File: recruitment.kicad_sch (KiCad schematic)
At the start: 1 part

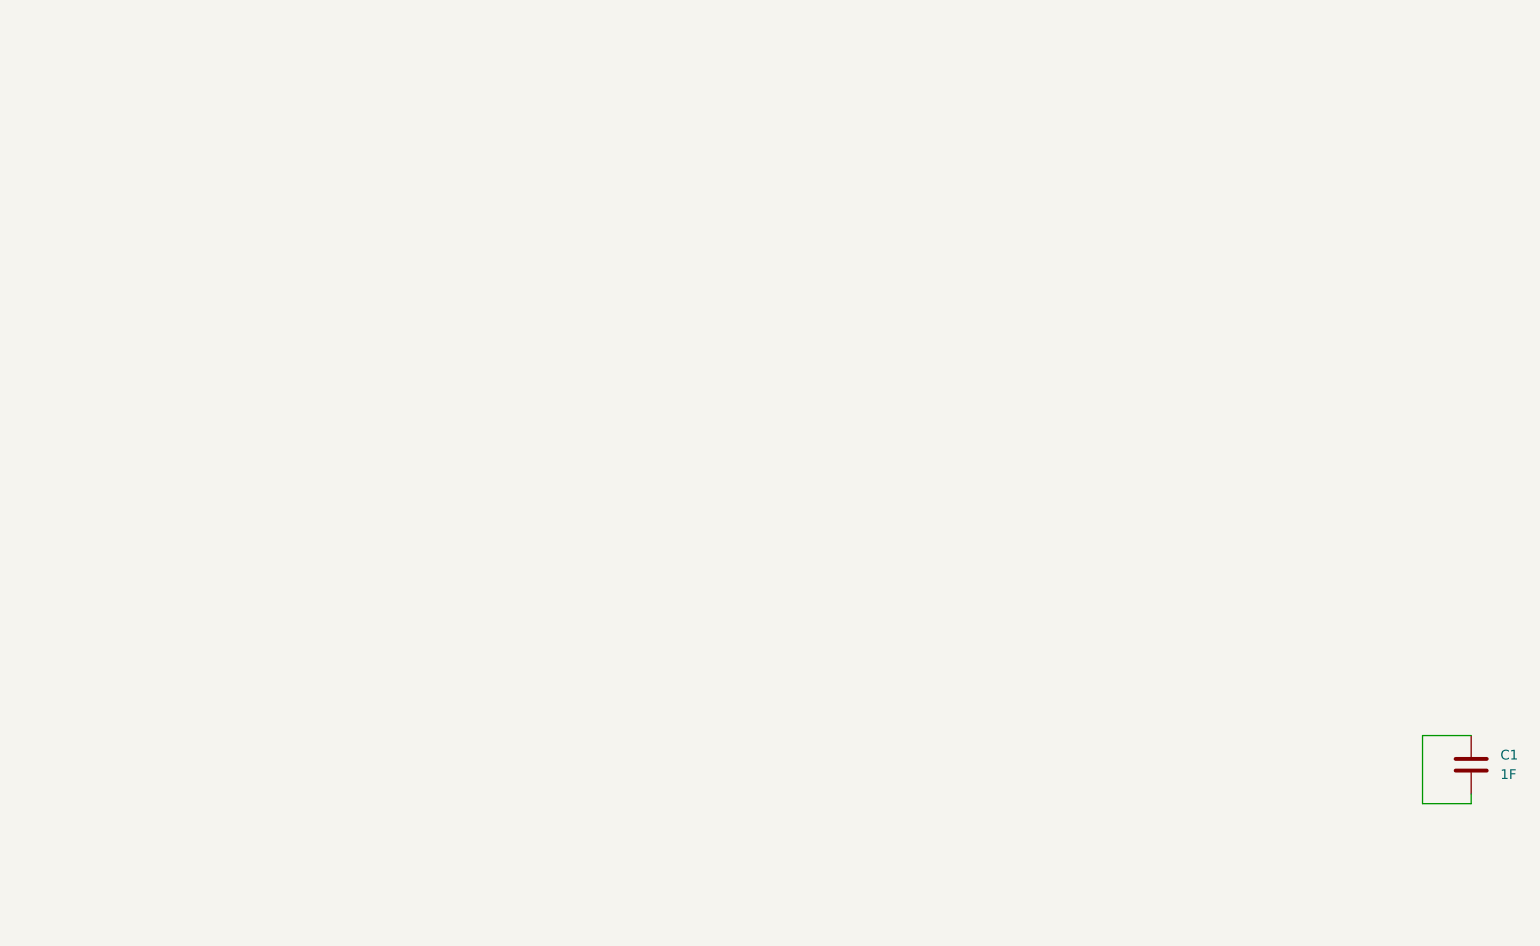
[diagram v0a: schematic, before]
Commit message: inizio progettazione circuito
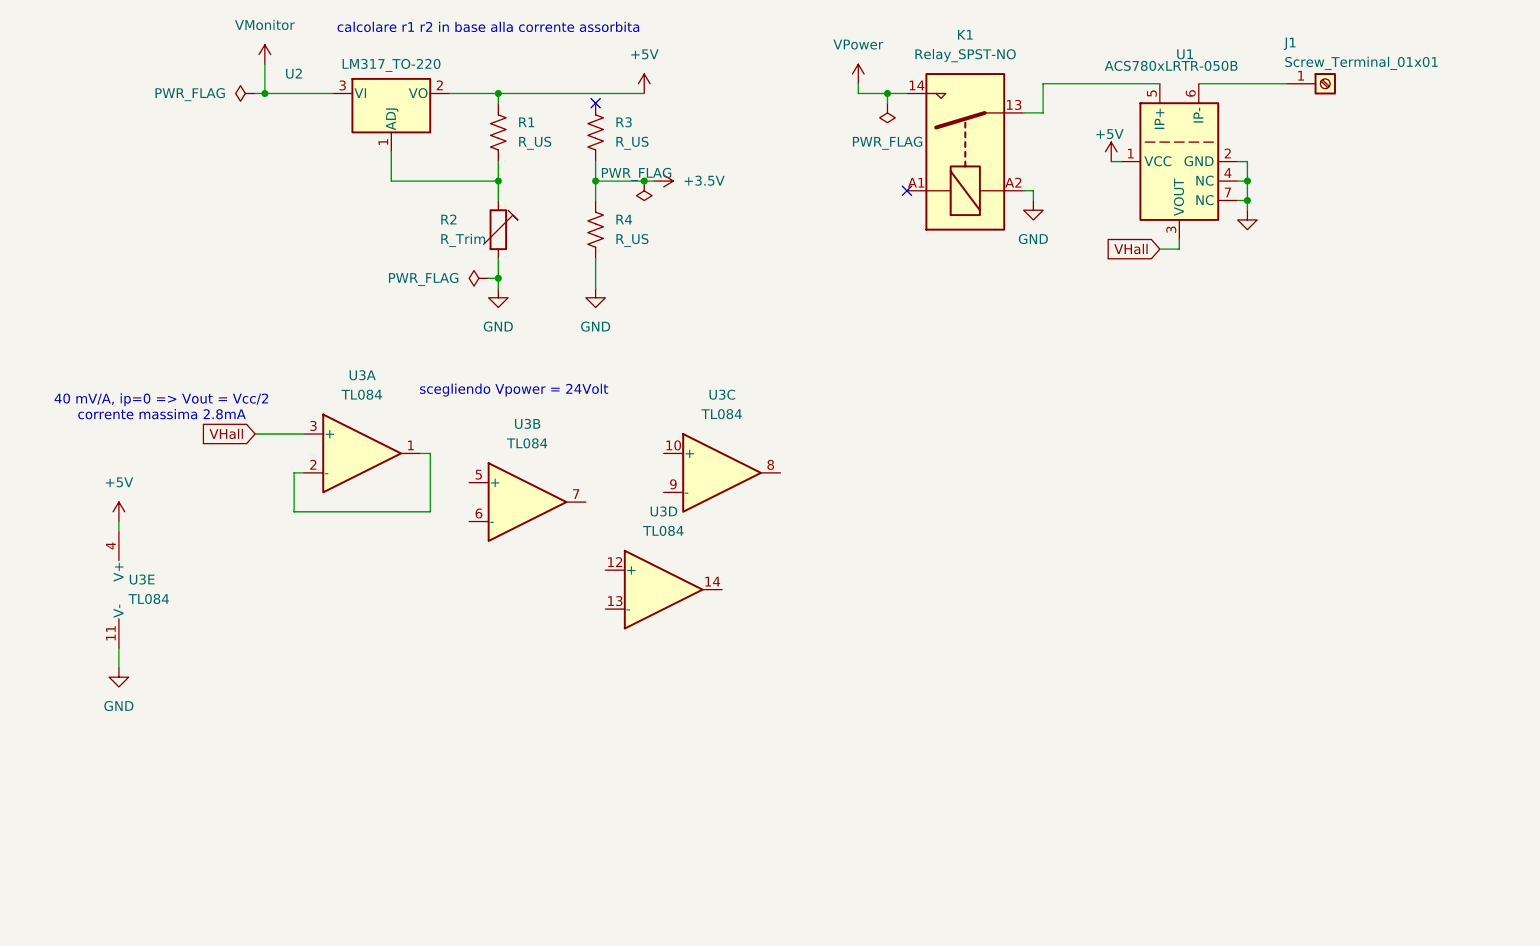
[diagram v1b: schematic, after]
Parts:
- removed C1: 1F, Capacitor_SMD:C_0805_2012Metric, symbol Device:C
- added J1: Screw_Terminal_01x01, TerminalBlock:TerminalBlock_Altech_AK300-2_P5.00mm, symbol Connector:Screw_Terminal_01x01
- added K1: Relay_SPST-NO, Relay_THT:Relay_1-Form-A_Schrack-RYII_RM5mm, symbol Relay:Relay_SPST-NO
- added R1, R3, R4: R_US, symbol Device:R_US
- added R2: R_Trim, symbol Device:R_Trim
- added U1: ACS780xLRTR-050B, Sensor_Current:Allegro_PSOF-7_4.8x6.4mm_P1.60mm, symbol Sensor_Current:ACS780xLRTR-050B
- added U2: LM317_TO-220, Package_TO_SOT_THT:TO-220-3_Vertical, symbol Regulator_Linear:LM317_TO-220
- added U3: TL084, symbol Amplifier_Operational:TL084
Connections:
- new net: R1.2, R2.1, U2.1 (ADJ)
- new net: J1.1 (Pin_1), U1.6 (IP-)
- new net: K1.13, U1.5 (IP+)
- new net: U3.1, U3.2 (-)
- new net +3.5V: R3.2, R4.1
- new net +5V: R1.1, U1.1 (VCC), U2.2 (VO), U3.4 (V+)
- new net GND: K1.A2, R2.2, R4.2, U1.2 (GND), U1.4 (NC), U1.7 (NC), U3.11 (V-)
- new net VHall: U1.3 (VOUT), U3.3 (+)
- new net VMonitor: U2.3 (VI)
- new net VPower: K1.14
- no-connect marks 0 -> 2
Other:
- note added: "40 mV/A, ip=0 => Vout = Vcc/2 corrente massima 2.8mA"
- note added: "calcolare r1 r2 in base alla corrente assorbita"
- note added: "scegliendo Vpower = 24Volt"

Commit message: giorno 2 : prime prove e footprint
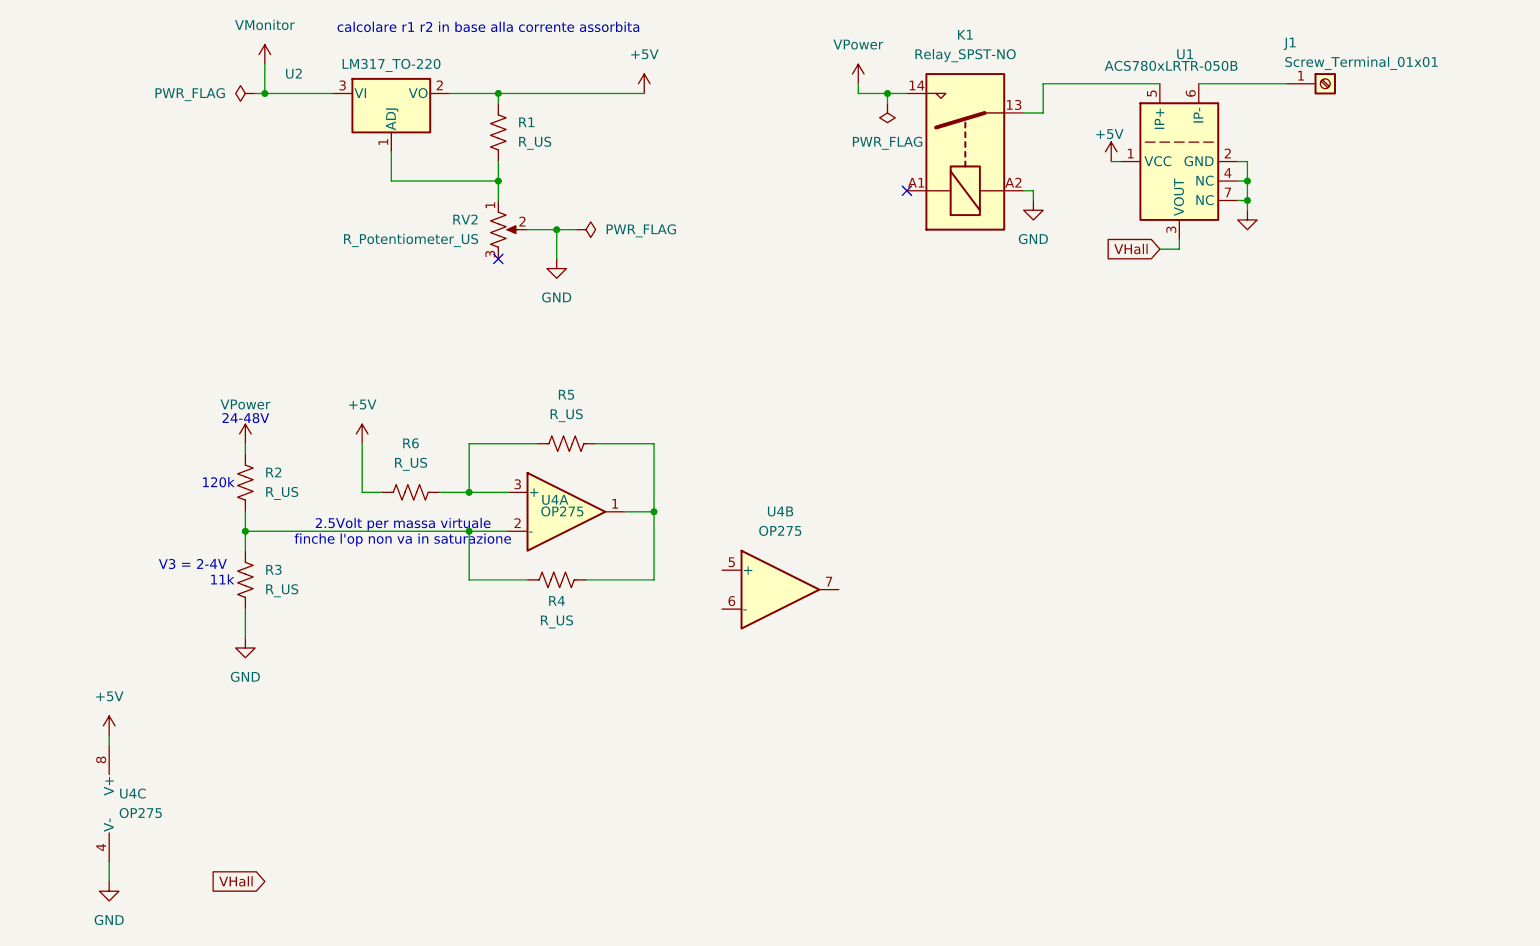
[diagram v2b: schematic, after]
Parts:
- removed R2: R_Trim, symbol Device:R_Trim
- removed U3: TL084, symbol Amplifier_Operational:TL084
- added R2, R5, R6: R_US, Resistor_THT:R_Axial_DIN0204_L3.6mm_D1.6mm_P2.54mm_Vertical, symbol Device:R_US
- added RV2: R_Potentiometer_US, Potentiometer_THT:Potentiometer_ACP_CA9-H2,5_Horizontal, symbol Device:R_Potentiometer_US
- added U4: OP275, symbol Amplifier_Operational:OP275
- R1, R3, R4: footprint (none) -> Resistor_THT:R_Axial_DIN0204_L3.6mm_D1.6mm_P2.54mm_Vertical
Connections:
- net +5V: now also R6.1, U4.8 (V+)
- net GND: now also R3.2, RV2.2, U4.4 (V-); no longer R4.2
- net VPower: now also R2.1
- net at R1.2, U2.1 (ADJ): now also RV2.1
- net at R3.1: now also R4.1, R2.2, U4.2 (-)
- removed net +3.5V: R3.2, R4.1
- new net: R4.2, R5.2, U4.1
- new net: R5.1, R6.2, U4.3 (+)
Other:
- note added: "11k"
- note added: "120k"
- note added: "2.5Volt per massa virtuale finche l'op non va in saturazione"
- note added: "24-48V"
- note added: "V3 = 2-4V"
- note removed: "40 mV/A, ip=0 => Vout = Vcc/2 corrente massima 2.8mA"
- note removed: "scegliendo Vpower = 24Volt"
